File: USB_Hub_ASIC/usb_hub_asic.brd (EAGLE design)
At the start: 101.6 x 50.8 mm, 105 parts, among them Q1 26M, SW1 RESET, U1 IC_MCP1603LT-330_3.3V_500MA_B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, U2 IC_CYUSB3314_QUAD_USB3.0_HUB, U3 IC_LM3674MF-1.2/NOPB_1.2V_600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

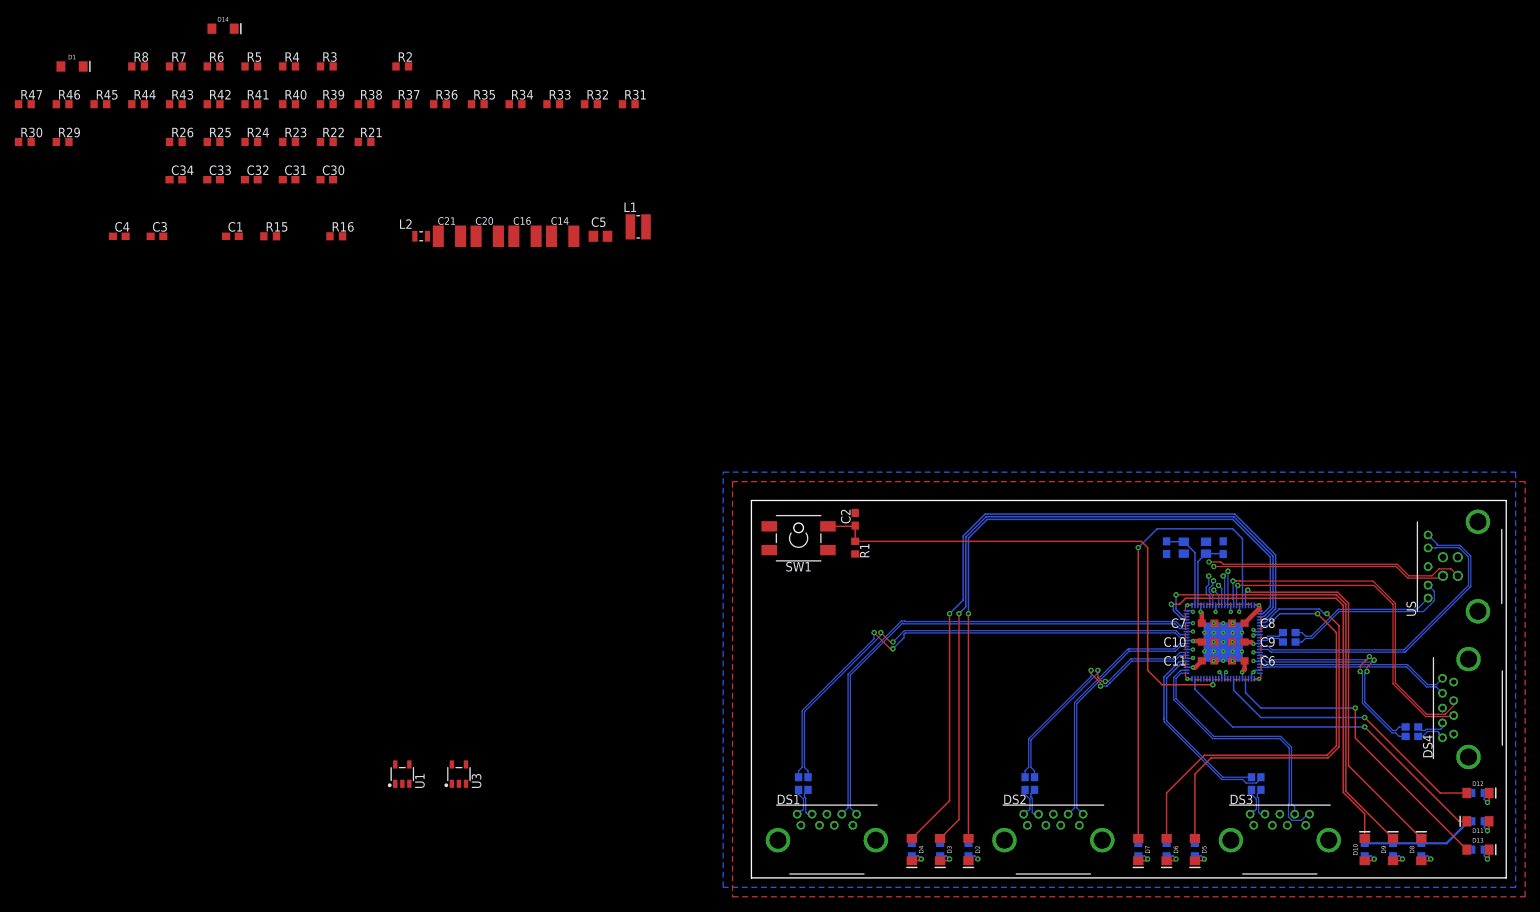
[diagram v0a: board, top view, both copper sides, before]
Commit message: ROUTING IS DONE?
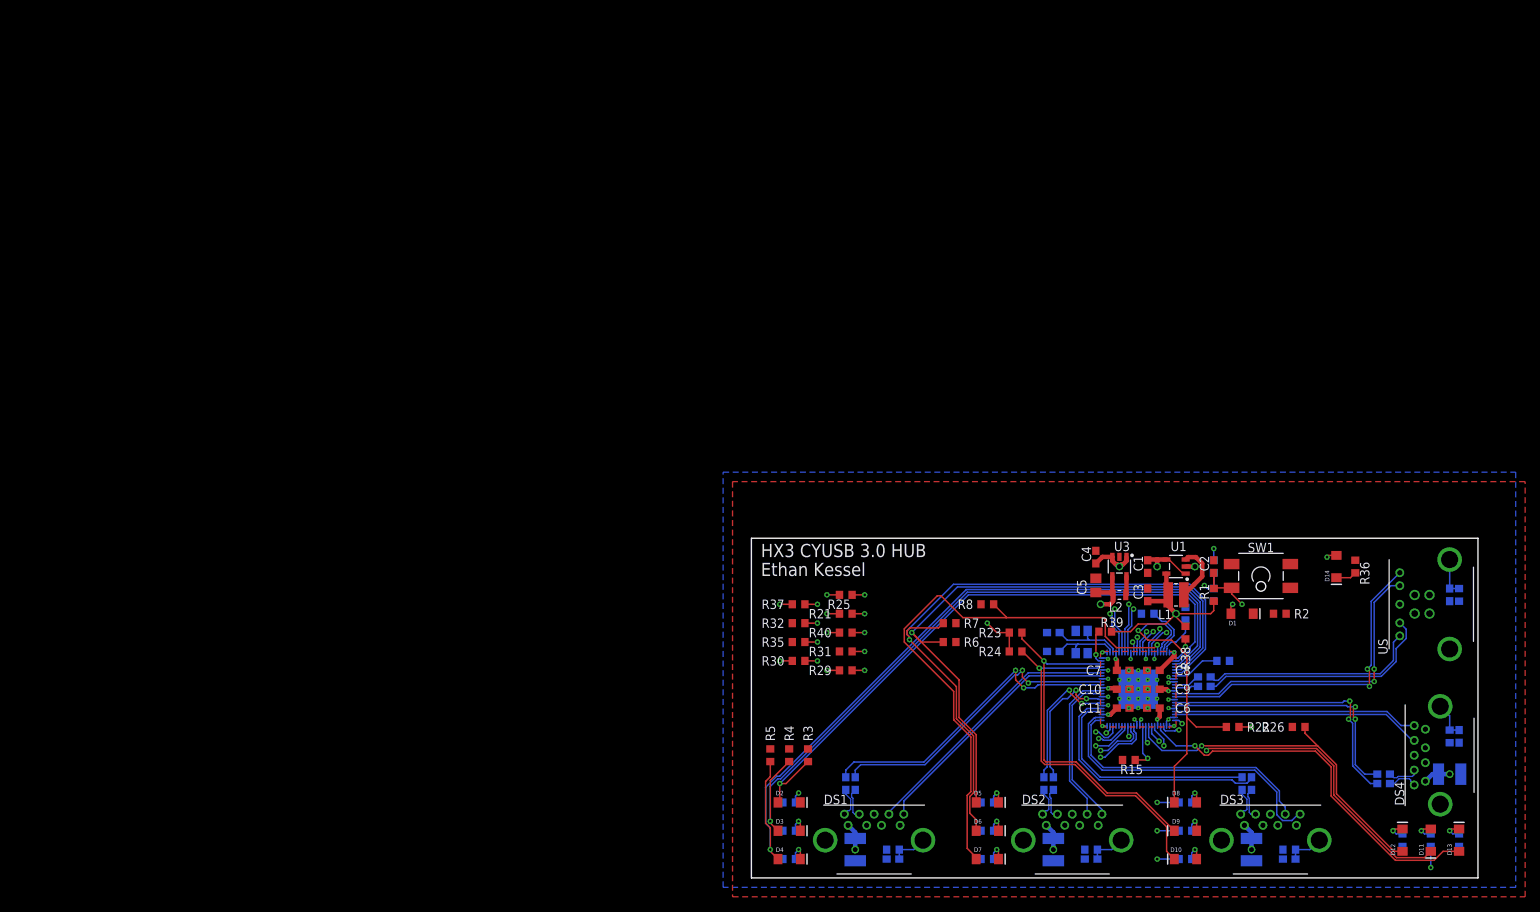
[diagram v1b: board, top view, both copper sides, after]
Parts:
- moved R45 200.6 mm to (94.0, 19.1), flipped to the bottom, turned to 90 degrees
- moved C34 188.3 mm to (95.2, 19.1), flipped to the bottom, turned to 270 degrees
- moved R44 184.6 mm to (72.4, 3.81), flipped to the bottom, turned to 180 degrees
- moved R41 175.5 mm to (95.2, 38.1), flipped to the bottom, turned to 90 degrees
- moved D1 173.9 mm to (66.0, 35.6)
- moved R47 173.1 mm to (62.2, 38.1), flipped to the bottom, turned to 270 degrees
- moved C33 171.2 mm to (72.4, 2.54), flipped to the bottom
- moved R26 170.4 mm to (73.7, 20.3), turned to 180 degrees
- moved R46 167.0 mm to (62.2, 41.9), flipped to the bottom, turned to 90 degrees
- moved D14 166.4 mm to (78.7, 41.9), turned to 270 degrees
- moved C30 161.1 mm to (94.0, 38.1), flipped to the bottom, turned to 270 degrees
- moved R43 158.9 mm to (45.7, 3.81), flipped to the bottom, turned to 180 degrees
- moved C21 152.8 mm to (94.0, 14.0), flipped to the bottom, turned to 180 degrees
- moved C32 145.4 mm to (45.7, 2.54), flipped to the bottom
- moved R22 145.1 mm to (64.8, 20.3)
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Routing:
- net +3V3: track 29.1 -> 303.3 mm, vias 8 -> 21
- net MODE_SEL[1]: track 0.00 -> 58.6 mm, vias 0 -> 2
- net MODE_SEL[0]: track 0.00 -> 57.9 mm, vias 0 -> 2
- net DS4_GREEN/VID_SEL[0]: track 45.4 -> 99.6 mm, vias 1 -> 3
- net DS4_PWREN/CDP_EN: track 0.00 -> 54.0 mm, vias 0 -> 2
- net DS1_PWREN/CDP_EN: track 0.00 -> 51.9 mm, vias 0 -> 2
- net DS1_OVRCURR: track 0.00 -> 51.5 mm, vias 0 -> 2
- net PWR_SW_POL: track 0.00 -> 50.7 mm, vias 0 -> 2
- net +5V: track 0.63 -> 50.2 mm, vias 1 -> 9
- net DS4_OVRCURR: track 0.00 -> 47.3 mm, vias 0 -> 2
- net US_OVRCURR: track 0.00 -> 45.6 mm, vias 0 -> 2
- net DS2_GREEN/NON_REMOVABLE[1]: track 58.9 -> 93.5 mm
- net DS1_RX_N: track 67.5 -> 35.4 mm
- net RESETIN: track 72.4 -> 40.3 mm, vias 1 -> 2
- net DS1_D_P: track 90.4 -> 59.0 mm
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- added copper zone on layer 15, net +5V
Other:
- board size 101.6 x 50.8 mm -> 97.8 x 45.7 mm
- board text added: "Ethan Kessel"
- board text added: "HX3 CYUSB 3.0 HUB"
